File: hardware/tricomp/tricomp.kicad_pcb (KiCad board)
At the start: 2 copper layers, 10 parts, among them J1 ISP, J2 Power/i2c, J3 Conn_01x05, J4 Conn_01x05, U1 ATMEGA328P-PU, Y1 Crystal

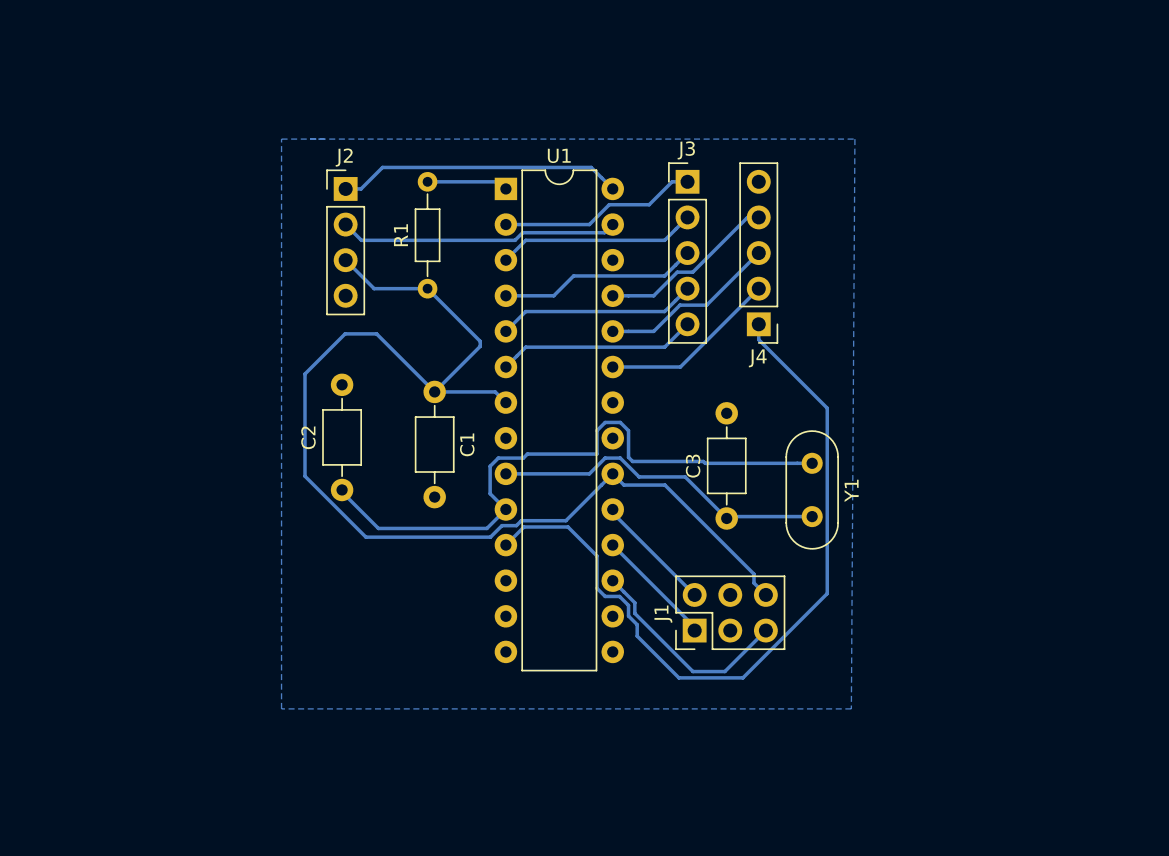
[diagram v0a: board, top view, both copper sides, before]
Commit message: building stripboard prototype
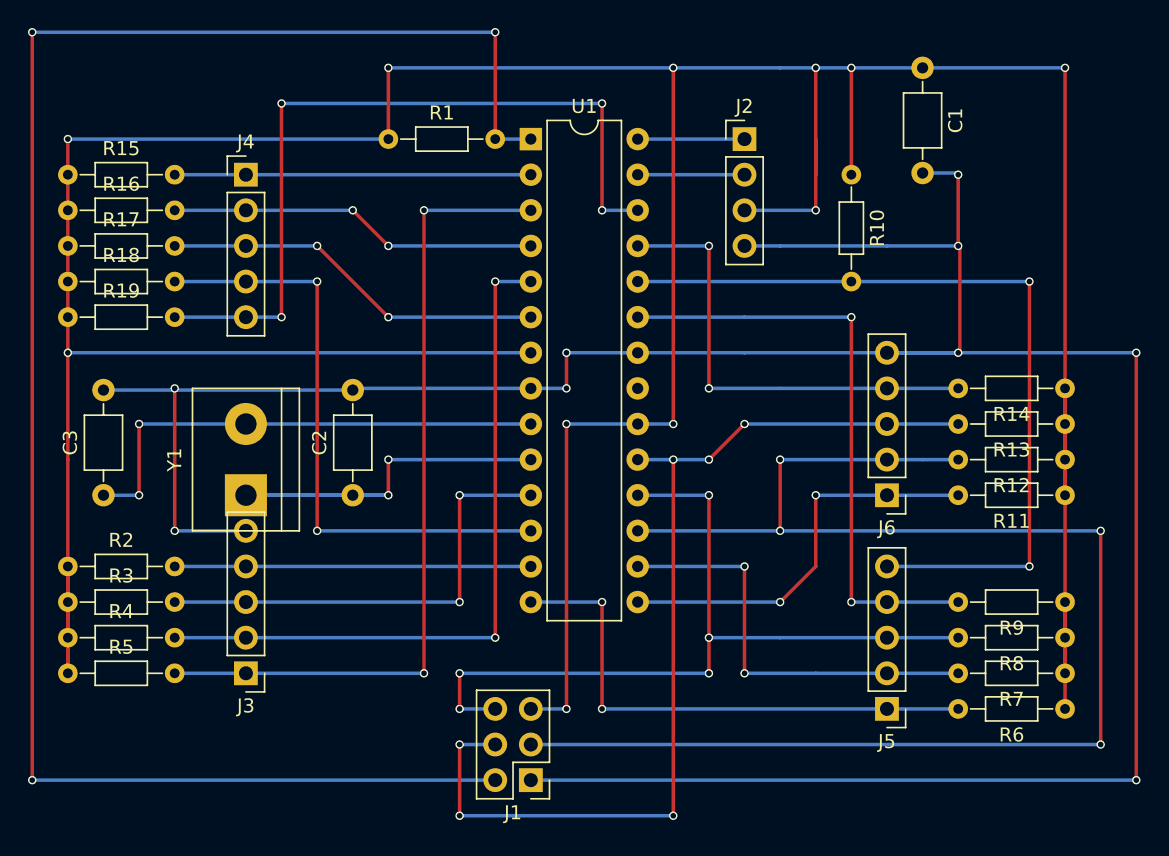
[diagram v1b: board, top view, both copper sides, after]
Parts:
- added J5: Conn_01x05, Pin_Headers:Pin_Header_Straight_1x05_Pitch2.54mm, F.Cu at (195.6, 139.7)
- added J6: Conn_01x05, Pin_Headers:Pin_Header_Straight_1x05_Pitch2.54mm, F.Cu at (195.6, 124.5)
- added R10: R, Resistors_THT:R_Axial_DIN0204_L3.6mm_D1.6mm_P7.62mm_Horizontal, F.Cu at (193.0, 101.6)
- added R11: R, Resistors_THT:R_Axial_DIN0204_L3.6mm_D1.6mm_P7.62mm_Horizontal, F.Cu at (208.3, 124.5)
- added R12: R, Resistors_THT:R_Axial_DIN0204_L3.6mm_D1.6mm_P7.62mm_Horizontal, F.Cu at (208.3, 121.9)
- added R13: R, Resistors_THT:R_Axial_DIN0204_L3.6mm_D1.6mm_P7.62mm_Horizontal, F.Cu at (208.3, 119.4)
- added R14: R, Resistors_THT:R_Axial_DIN0204_L3.6mm_D1.6mm_P7.62mm_Horizontal, F.Cu at (208.3, 116.8)
- added R15: R, Resistors_THT:R_Axial_DIN0204_L3.6mm_D1.6mm_P7.62mm_Horizontal, F.Cu at (137.2, 101.6)
- added R16: R, Resistors_THT:R_Axial_DIN0204_L3.6mm_D1.6mm_P7.62mm_Horizontal, F.Cu at (137.2, 104.1)
- added R17: R, Resistors_THT:R_Axial_DIN0204_L3.6mm_D1.6mm_P7.62mm_Horizontal, F.Cu at (137.2, 106.7)
- added R18: R, Resistors_THT:R_Axial_DIN0204_L3.6mm_D1.6mm_P7.62mm_Horizontal, F.Cu at (137.2, 109.2)
- added R19: R, Resistors_THT:R_Axial_DIN0204_L3.6mm_D1.6mm_P7.62mm_Horizontal, F.Cu at (137.2, 111.8)
- added R2: R, Resistors_THT:R_Axial_DIN0204_L3.6mm_D1.6mm_P7.62mm_Horizontal, F.Cu at (137.2, 129.5)
- added R3: R, Resistors_THT:R_Axial_DIN0204_L3.6mm_D1.6mm_P7.62mm_Horizontal, F.Cu at (137.2, 132.1)
- added R4: R, Resistors_THT:R_Axial_DIN0204_L3.6mm_D1.6mm_P7.62mm_Horizontal, F.Cu at (137.2, 134.6)
- added R5: R, Resistors_THT:R_Axial_DIN0204_L3.6mm_D1.6mm_P7.62mm_Horizontal, F.Cu at (137.2, 137.2)
- added R6: R, Resistors_THT:R_Axial_DIN0204_L3.6mm_D1.6mm_P7.62mm_Horizontal, F.Cu at (208.3, 139.7)
- added R7: R, Resistors_THT:R_Axial_DIN0204_L3.6mm_D1.6mm_P7.62mm_Horizontal, F.Cu at (208.3, 137.2)
- added R8: R, Resistors_THT:R_Axial_DIN0204_L3.6mm_D1.6mm_P7.62mm_Horizontal, F.Cu at (208.3, 134.6)
- added R9: R, Resistors_THT:R_Axial_DIN0204_L3.6mm_D1.6mm_P7.62mm_Horizontal, F.Cu at (208.3, 132.1)
- Y1: footprint Crystals:Crystal_HC52-8mm_Vertical -> Connectors_Terminal_Blocks:TerminalBlock_bornier-2_P5.08mm
- moved J3 47.1 mm to (149.9, 137.2), turned to 180 degrees
- moved C3 44.5 mm to (139.7, 124.5)
- moved C1 41.8 mm to (198.1, 94.0)
- moved Y1 40.5 mm to (149.9, 124.5), turned to 90 degrees
- moved J4 38.1 mm to (149.9, 101.6), turned to 0 degrees
- moved J2 28.7 mm to (185.4, 99.1)
- moved J1 15.8 mm to (170.2, 144.8), turned to 180 degrees
- moved R1 11.0 mm to (160.0, 99.1), turned to 0 degrees
- moved U1 3.98 mm to (170.2, 99.1)
- moved C2 0.85 mm to (157.5, 124.5)
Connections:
- J1 pad 1: Net-(J1-Pad1) -> Earth
- J1 pad 4: Earth -> Net-(J1-Pad4)
- J1 pad 5: Net-(J1-Pad5) -> +5V
- J1 pad 6: +5V -> Net-(J1-Pad6)
- J3 pad 5: Net-(J3-Pad5) -> Earth
- J4 pad 5: Earth -> Net-(J4-Pad5)
- R1 pad 2: Net-(J1-Pad3) -> Net-(J1-Pad2)
- U1 pad 1: Net-(J1-Pad3) -> Net-(J1-Pad2)
- U1 pad 11: Net-(J4-Pad1) -> Net-(J3-Pad3)
- U1 pad 12: (no net) -> Net-(J4-Pad4)
- U1 pad 13: (no net) -> Net-(J3-Pad4)
- U1 pad 14: (no net) -> Net-(J5-Pad1)
- U1 pad 15: (no net) -> Net-(J6-Pad1)
- U1 pad 16: (no net) -> Net-(J5-Pad2)
- U1 pad 17: Net-(J1-Pad5) -> Net-(J1-Pad3)
- U1 pad 18: Net-(J1-Pad1) -> Net-(J1-Pad6)
- U1 pad 19: Net-(J1-Pad2) -> Net-(J1-Pad4)
- U1 pad 2: Net-(J3-Pad1) -> Net-(J4-Pad1)
- U1 pad 23: Net-(J4-Pad2) -> Net-(J5-Pad4)
- U1 pad 24: Net-(J4-Pad3) -> Net-(J5-Pad5)
- U1 pad 25: Net-(J4-Pad4) -> Net-(J6-Pad4)
- U1 pad 26: (no net) -> Net-(J4-Pad5)
- U1 pad 3: Net-(J3-Pad2) -> Net-(J3-Pad1)
- U1 pad 4: Net-(J3-Pad3) -> Net-(J4-Pad2)
- U1 pad 5: Net-(J3-Pad4) -> Net-(J3-Pad2)
- U1 pad 6: Net-(J3-Pad5) -> Net-(J4-Pad3)
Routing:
- net +5V: track 82.3 -> 294.6 mm, vias 0 -> 11
- net Earth: track 0.36 -> 201.3 mm, vias 0 -> 10
- net Net-(J1-Pad2): track 8.52 -> 129.5 mm, vias 0 -> 3
- net Net-(J1-Pad3): track 5.80 -> 106.7 mm, vias 0 -> 4
- net Net-(J1-Pad4): track 0.00 -> 72.2 mm, vias 0 -> 6
- net Net-(J5-Pad5): track 0.00 -> 58.4 mm, vias 0 -> 2
- net Net-(J1-Pad6): track 0.00 -> 58.4 mm, vias 0 -> 5
- net Net-(J4-Pad5): track 0.00 -> 55.9 mm, vias 0 -> 4
- net Net-(J3-Pad1): track 14.2 -> 58.4 mm, vias 0 -> 2
- net Net-(J5-Pad4): track 0.00 -> 43.2 mm, vias 0 -> 2
- net Net-(J5-Pad1): track 0.00 -> 38.1 mm, vias 0 -> 2
- net Net-(J3-Pad2): track 14.2 -> 50.8 mm, vias 0 -> 2
- net Net-(J6-Pad4): track 0.00 -> 33.0 mm, vias 0 -> 2
- net Net-(J5-Pad2): track 0.00 -> 30.5 mm, vias 0 -> 2
- net Net-(J4-Pad4): track 12.7 -> 43.2 mm, vias 0 -> 2
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- removed copper zone on B.Cu, net Earth
